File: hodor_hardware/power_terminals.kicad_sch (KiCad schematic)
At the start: 56 parts, among them J1 Screw_Terminal_01x02, Q1 SiS443DN, T1 GND, T10 V_{BUS}, T12 5V, T14 V_{BUS}_SENSE, T32 GND, T6 V_{DC}_SENSE, T9 V_{DC}, U5 TPS54240DRC

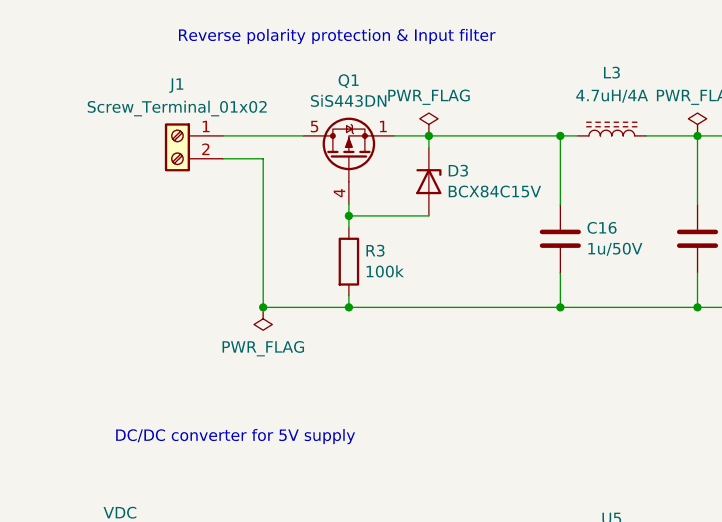
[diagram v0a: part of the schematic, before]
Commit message: Latest changes
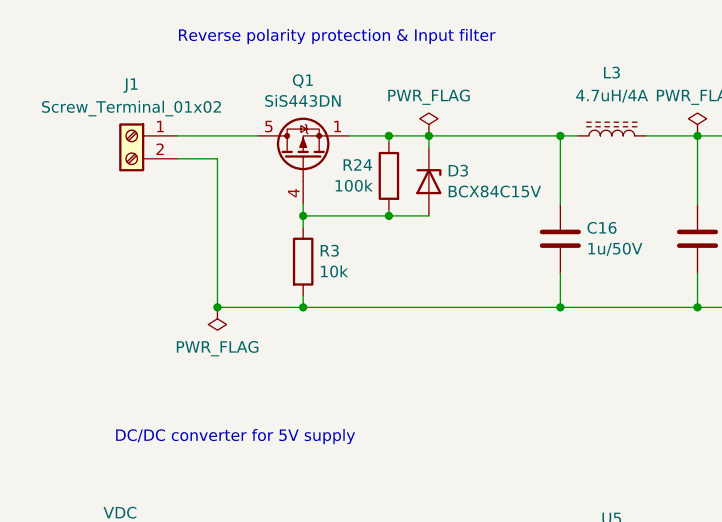
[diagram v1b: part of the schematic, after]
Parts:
- added R24: 100k, Resistor_SMD:R_0402_1005Metric, symbol Device:R
- R3: value 100k -> 10k
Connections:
- net at C16.1, D3.1 (K), L3.1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: now also R24.1
- net at D3.2 (A), Q1.4 (G), R3.1: now also R24.2
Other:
- moved on the sheet: J1, Q1, R3
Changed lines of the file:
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@@
 	)
 	(junction
-		(at 48.26 40.005)
+		(at 43.18 40.005)
 		(diameter 0)
 		(color 0 0 0 0)
@@
 	)
 	(junction
-		(at 38.735 50.165)
+		(at 33.655 50.165)
 		(diameter 0)
 		(color 0 0 0 0)
@@
 	)
 	(junction
+		(at 52.705 31.115)
+		(diameter 0)
+		(color 0 0 0 0)
+	)
+	(junction
 		(at 71.755 31.115)
 		(diameter 0)
@@
 	)
 	(junction
-		(at 48.26 50.165)
+		(at 43.18 50.165)
+		(diameter 0)
+		(color 0 0 0 0)
+	)
+	(junction
+		(at 52.705 40.005)
 		(diameter 0)
 		(color 0 0 0 0)
@@
 	(wire
 		(pts
-			(xy 38.735 50.165) (xy 48.26 50.165)
+			(xy 33.655 50.165) (xy 43.18 50.165)
 		)
 		(stroke
@@
 	(wire
 		(pts
+			(xy 52.705 40.005) (xy 57.15 40.005)
+		)
+		(stroke
+			(width 0)
+			(type default)
+		)
+	)
+	(wire
+		(pts
+			(xy 52.705 31.115) (xy 57.15 31.115)
+		)
+		(stroke
+			(width 0)
+			(type default)
+		)
+	)
+	(wire
+		(pts
+			(xy 52.705 39.37) (xy 52.705 40.005)
+		)
+		(stroke
+			(width 0)
+			(type default)
+		)
+	)
+	(wire
+		(pts
 			(xy 102.87 171.45) (xy 102.87 170.18)
 		)
@@
 	(wire
 		(pts
-			(xy 34.29 33.655) (xy 38.735 33.655)
+			(xy 29.21 33.655) (xy 33.655 33.655)
 		)
 		(stroke
@@
 	(wire
 		(pts
-			(xy 38.735 33.655) (xy 38.735 50.165)
+			(xy 33.655 33.655) (xy 33.655 50.165)
 		)
 		(stroke
@@
 	(wire
 		(pts
+			(xy 52.705 31.115) (xy 52.705 31.75)
+		)
+		(stroke
+			(width 0)
+			(type default)
+		)
+	)
+	(wire
+		(pts
 			(xy 99.695 31.115) (xy 99.695 38.735)
 		)
@@
 	(wire
 		(pts
-			(xy 48.26 40.005) (xy 57.15 40.005)
+			(xy 43.18 40.005) (xy 52.705 40.005)
 		)
 		(stroke
@@
 	(wire
 		(pts
-			(xy 34.29 31.115) (xy 43.18 31.115)
+			(xy 29.21 31.115) (xy 38.1 31.115)
 		)
 		(stroke
@@
 	(wire
 		(pts
-			(xy 48.26 40.005) (xy 48.26 41.275)
+			(xy 43.18 40.005) (xy 43.18 41.275)
 		)
 		(stroke
@@
 	(wire
 		(pts
-			(xy 48.26 38.735) (xy 48.26 40.005)
+			(xy 43.18 38.735) (xy 43.18 40.005)
 		)
 		(stroke
@@
 	(wire
 		(pts
-			(xy 48.26 50.165) (xy 48.26 48.895)
+			(xy 43.18 50.165) (xy 43.18 48.895)
 		)
 		(stroke
@@
 	(wire
 		(pts
-			(xy 48.26 50.165) (xy 71.755 50.165)
+			(xy 43.18 50.165) (xy 71.755 50.165)
 		)
 		(stroke
@@
 	(wire
 		(pts
-			(xy 53.34 31.115) (xy 57.15 31.115)
+			(xy 48.26 31.115) (xy 52.705 31.115)
 		)
 		(stroke
@@
 	(symbol
 		(lib_id "Transistor_FET:SiS443DN")
-		(at 48.26 33.655 90)
+		(at 43.18 33.655 90)
 		(unit 1)
 		(exclude_from_sim no)
@@
 		(dnp no)
 		(property "Reference" "Q1"
-			(at 48.26 24.9682 90)
+			(at 43.18 24.9682 90)
 			(effects
 				(font
@@
 		)
 		(property "Value" "SiS443DN"
-			(at 48.26 27.2796 90)
+			(at 43.18 27.2796 90)
 			(effects
 				(font
@@
 		)
 		(property "Footprint" "Package_SO:Vishay_PowerPAK_1212-8_Single"
-			(at 50.165 28.575 0)
+			(at 45.085 28.575 0)
 			(effects
 				(font
@@
 		)
 		(property "Datasheet" "https://www.vishay.com/docs/63253/sis443dn.pdf"
-			(at 48.26 33.655 90)
+			(at 43.18 33.655 90)
 			(effects
 				(font
@@
 		)
 		(property "Description" "-35A Id, -40V Vds, P-Channel MOSFET, PowerPAK 1212-8 Single"
-			(at 48.26 33.655 0)
+			(at 43.18 33.655 0)
 			(effects
 				(font
@@
 	(symbol
 		(lib_id "Device:R")
-		(at 48.26 45.085 0)
+		(at 43.18 45.085 0)
 		(unit 1)
 		(exclude_from_sim no)
@@
 		(dnp no)
 		(property "Reference" "R3"
-			(at 50.038 43.9166 0)
+			(at 44.958 43.9166 0)
 			(effects
 				(font
@@
 			)
 		)
-		(property "Value" "100k"
-			(at 50.038 46.228 0)
+		(property "Value" "10k"
+			(at 44.958 46.228 0)
 			(effects
 				(font
@@
 		)
 		(property "Footprint" "Resistor_SMD:R_0402_1005Metric"
-			(at 46.482 45.085 90)
+			(at 41.402 45.085 90)
 			(effects
 				(font
@@
 		)
 		(property "Datasheet" "~"
-			(at 48.26 45.085 0)
+			(at 43.18 45.085 0)
 			(effects
 				(font
@@
 		)
 		(property "Description" "Resistor"
-			(at 48.26 45.085 0)
+			(at 43.18 45.085 0)
 			(effects
 				(font
@@
 	(symbol
 		(lib_id "Connector:Screw_Terminal_01x02")
-		(at 29.21 31.115 0)
+		(at 24.13 31.115 0)
 		(mirror y)
 		(unit 1)
@@
 		(fields_autoplaced yes)
 		(property "Reference" "J1"
-			(at 29.21 25.4 0)
+			(at 24.13 25.4 0)
 			(effects
 				(font
@@
 		)
 		(property "Value" "Screw_Terminal_01x02"
-			(at 29.21 27.94 0)
+			(at 24.13 27.94 0)
 			(effects
 				(font
@@
 		)
 		(property "Footprint" "TerminalBlock_Phoenix:TerminalBlock_Phoenix_MKDS-1,5-2_1x02_P5.00mm_Horizontal"
-			(at 29.21 31.115 0)
+			(at 24.13 31.115 0)
 			(effects
 				(font
@@
 		)
 		(property "Datasheet" "~"
-			(at 29.21 31.115 0)
+			(at 24.13 31.115 0)
 			(effects
 				(font
@@
 		)
 		(property "Description" "Generic screw terminal, single row, 01x02, script generated (kicad-library-utils/schlib/autogen/connector/)"
-			(at 29.21 31.115 0)
+			(at 24.13 31.115 0)
 			(effects
 				(font
@@
 	)
 	(symbol
+		(lib_id "Device:R")
+		(at 52.705 35.56 0)
+		(mirror y)
+		(unit 1)
+		(exclude_from_sim no)
+		(in_bom yes)
+		(on_board yes)
+		(dnp no)
+		(property "Reference" "R24"
+			(at 50.927 34.3916 0)
+			(effects
+				(font
+					(size 1.27 1.27)
+				)
+				(justify left)
+			)
+		)
+		(property "Value" "100k"
+			(at 50.927 36.703 0)
+			(effects
+				(font
+					(size 1.27 1.27)
+				)
+				(justify left)
+			)
+		)
+		(property "Footprint" "Resistor_SMD:R_0402_1005Metric"
+			(at 54.483 35.56 90)
+			(effects
+				(font
+					(size 1.27 1.27)
+				)
+				(hide yes)
+			)
+		)
+		(property "Datasheet" "~"
+			(at 52.705 35.56 0)
+			(effects
+				(font
+					(size 1.27 1.27)
+				)
+				(hide yes)
+			)
+		)
+		(property "Description" "Resistor"
+			(at 52.705 35.56 0)
+			(effects
+				(font
+					(size 1.27 1.27)
+				)
+				(hide yes)
+			)
+		)
+		(pin "1"
+		)
+		(pin "2"
+		)
+		(instances
+			(project "hodor_hardware"
+				(path "/2da01e60-41ef-423d-82f4-a5c8908d8b96/4a2ab631-9c09-4ff5-b76c-afe5090e4ede"
+					(reference "R24")
+					(unit 1)
+				)
+			)
+		)
+	)
+	(symbol
 		(lib_id "power:GND")
 		(at 83.82 181.61 0)
@@
 	(symbol
 		(lib_id "power:PWR_FLAG")
-		(at 38.735 50.165 180)
+		(at 33.655 50.165 180)
 		(unit 1)
 		(exclude_from_sim no)
@@
 		(fields_autoplaced yes)
 		(property "Reference" "#FLG03"
-			(at 38.735 52.07 0)
+			(at 33.655 52.07 0)
 			(effects
 				(font
@@
 		)
 		(property "Value" "PWR_FLAG"
-			(at 38.735 54.61 0)
+			(at 33.655 54.61 0)
 			(effects
 				(font
@@
 		)
 		(property "Footprint" ""
-			(at 38.735 50.165 0)
+			(at 33.655 50.165 0)
 			(effects
 				(font
@@
 		)
 		(property "Datasheet" "~"
-			(at 38.735 50.165 0)
+			(at 33.655 50.165 0)
 			(effects
 				(font
@@
 		)
 		(property "Description" "Special symbol for telling ERC where power comes from"
-			(at 38.735 50.165 0)
+			(at 33.655 50.165 0)
 			(effects
 				(font
